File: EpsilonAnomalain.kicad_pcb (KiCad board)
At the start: 4 copper layers, 55 x 55 mm, 99 parts, among them J1 USB_C, J2 I2C, J3 ServoA, J4 ServoB, J5 ServoC, J6 ServoD, J7 UART, J8 Power, Q1 BC817-40, SW1 TS-1187A-B-A-B, SW2 TS-1187A-B-A-B, SW3 TS-1187A-B-A-B, U1 AP2112K-3.3, U10 W25N01GVZEIG, U2 TPS61088, U3 USBLC6-2SC6, U4 ESP32-S3FN8, U5 ICM-42688-P, U6 AHT20, U7 BMP388, U8 SS206SURWA/S530-A3/S290, U9 74HC595, Y1 40 MHz

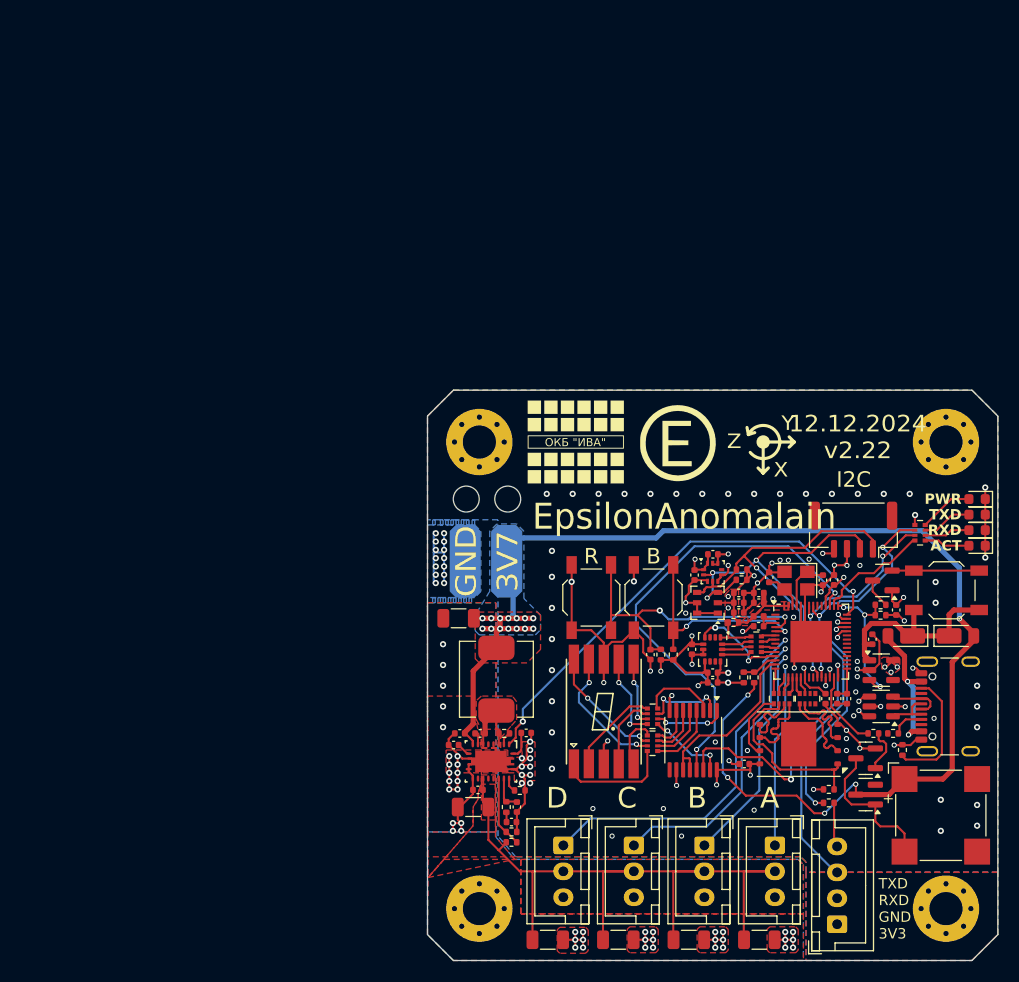
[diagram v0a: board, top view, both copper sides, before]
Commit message: update
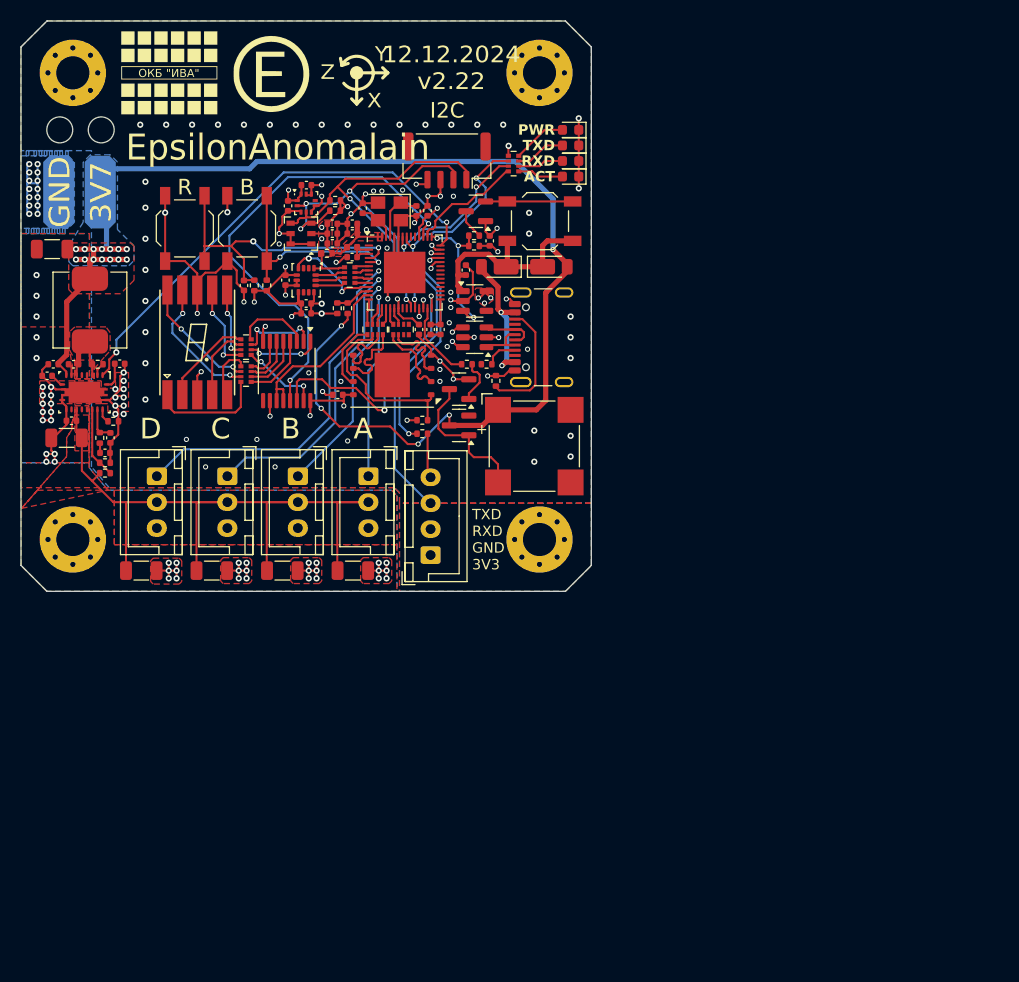
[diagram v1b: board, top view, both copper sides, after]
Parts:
- moved C14 53.0 mm to (193.2, 78.6)
- moved C18 53.0 mm to (197.4, 78.6)
- moved D1 53.0 mm to (234.7, 62.1)
- moved G*** 53.0 mm to (203.1, 43.4)
- moved J5 53.0 mm to (208.7, 82.3)
- moved J8 53.0 mm to (190.5, 58.9)
- moved L1 53.0 mm to (220.7, 60.2)
- moved R11 53.0 mm to (219.1, 56.7)
- moved R8 53.0 mm to (234.6, 73.1)
- moved REF** 53.0 mm to (213.0, 43.3)
- moved SW2 53.0 mm to (204.6, 58.4)
- moved SW3 53.0 mm to (210.6, 58.4)
- moved U10 53.0 mm to (224.6, 72.5)
- moved C17 53.0 mm to (191.9, 71.5)
- moved C19 53.0 mm to (198.3, 71.5)
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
